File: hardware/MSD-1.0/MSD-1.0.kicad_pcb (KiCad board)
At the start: 2 copper layers, 98.4 x 44.4 mm, 27 parts, among them J1 Conn_01x05, J2 Conn_01x03, Q1 IRF840, U1 NE555P, U2 PC817, U3 PC817

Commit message: new file:   .~BoM.xlsx 	new file:   BoM.xlsx 	new file:   hardware/BoM.xlsx 	deleted:    hardware/MSD-1.0/MSD-1.0-backups/MSD-1.0-2025-03-26_092035.zip 	deleted:    hardware/MSD-1.0/MSD-1.0-backups/MSD-1.0-2025-03-26_092834.zip 	deleted:    hardware/MSD-1.0/MSD-1.0-backups/MSD-1.0-2025-03-27_092014.zip 	new file:   hardware/MSD-1.0/MSD-1.0-backups/MSD-1.0-2025-04-28_130614.zip 	new file:   hardware/MSD-1.0/MSD-1.0-backups/MSD-1.0-2025-04-28_131128.zip 	new file:   hardware/MSD-1.0/MSD-1.0-backups/MSD-1.0-2025-04-28_132753.zip 	new file:   hardware/MSD-1.0/MSD-1.0.csv 	modified:   hardware/MSD-1.0/MSD-1.0.kicad_pcb 	modified:   hardware/MSD-1.0/MSD-1.0.kicad_sch 	deleted:    hardware/PS-1.0/PS-1.0-backups/PS-1.0-2025-03-24_111800.zip 	deleted:    hardware/PS-1.0/PS-1.0-backups/PS-1.0-2025-03-24_112738.zip 	deleted:    hardware/PS-1.0/PS-1.0-backups/PS-1.0-2025-03-25_152833.zip 	deleted:    hardware/PS-1.0/PS-1.0-backups/PS-1.0-2025-03-25_154601.zip 	deleted:    hardware/PS-1.0/PS-1.0-backups/PS-1.0-2025-03-25_155821.zip 	deleted:    hardware/PS-1.0/PS-1.0-backups/PS-1.0-2025-04-11_101418.zip 	deleted:    hardware/PS-1.0/PS-1.0-backups/PS-1.0-2025-04-11_110528.zip 	deleted:    hardware/PS-1.0/PS-1.0-backups/PS-1.0-2025-04-11_111527.zip 	deleted:    hardware/PS-1.0/PS-1.0-backups/PS-1.0-2025-04-11_114252.zip 	deleted:    hardware/PS-1.0/PS-1.0-backups/PS-1.0-2025-04-17_105409.zip 	new file:   hardware/PS-1.0/PS-1.0-backups/PS-1.0-2025-04-19_071925.zip 	new file:   hardware/PS-1.0/PS-1.0-backups/PS-1.0-2025-04-27_222808.zip 	new file:   hardware/PS-1.0/PS-1.0-backups/PS-1.0-2025-04-27_223939.zip 	new file:   hardware/PS-1.0/PS-1.0-backups/PS-1.0-2025-04-27_224445.zip 	new file:   hardware/PS-1.0/PS-1.0-backups/PS-1.0-2025-04-27_225206.zip 	new file:   hardware/PS-1.0/PS-1.0-backups/PS-1.0-2025-04-27_230217.zip 	new file:   hardware/PS-1.0/PS-1.0-backups/PS-1.0-2025-04-28_083014.zip 	new file:   hardware/PS-1.0/PS-1.0-backups/PS-1.0-2025-04-28_112951.zip 	new file:   har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
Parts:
- C1: value 2.2nF -> 2.2nF 100
- C2: value 10nF -> 10nF 63
- C3: value 0.022uF 400V MKP -> 0.022uF 400
- C4: value 100nF -> 100nF 100
- C5: value 100nF 400V -> 100nF 400
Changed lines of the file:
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@@
 			)
 		)
-		(property "Value" "10nF"
+		(property "Value" "10nF 63"
 			(at 2.5 3 0)
 			(layer "F.Fab")
@@
 			)
 		)
-		(property "Value" "0.022uF 400V MKP"
+		(property "Value" "0.022uF 400"
 			(at 5 3.75 0)
 			(layer "F.Fab")
@@
 			)
 		)
-		(property "Value" "100nF 400V"
+		(property "Value" "100nF 400"
 			(at 5 3.75 0)
 			(layer "F.Fab")
@@
 			)
 		)
-		(property "Value" "100nF"
+		(property "Value" "100nF 100"
 			(at 2.5 3 0)
 			(layer "F.Fab")
@@
 			)
 		)
-		(property "Value" "2.2nF"
+		(property "Value" "2.2nF 100"
 			(at 2.5 3 0)
 			(layer "F.Fab")

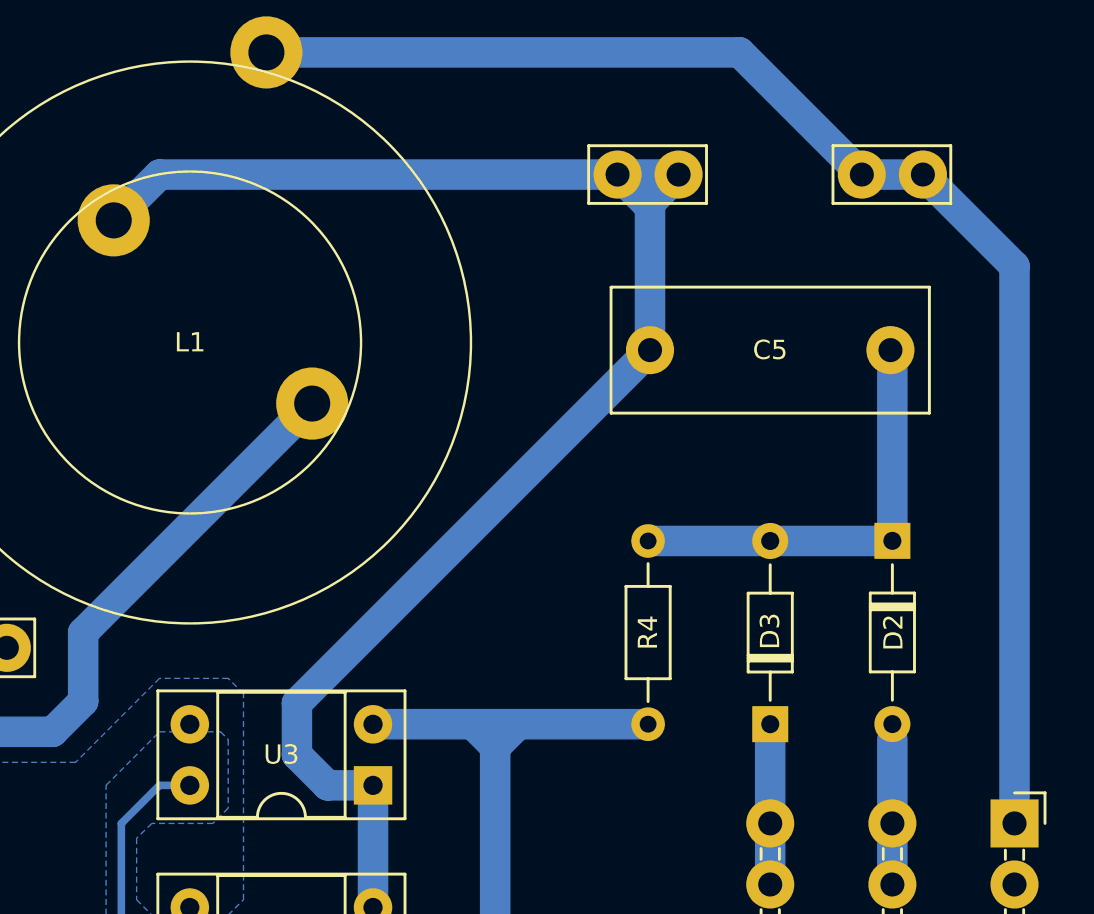
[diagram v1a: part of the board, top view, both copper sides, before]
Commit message: modified:   .DS_Store 	modified:   README.md 	deleted:    hardware/MSD-1.0/MSD-1.0 BoM.csv 	deleted:    hardware/MSD-1.0/MSD-1.0-backups/MSD-1.0-2025-04-08_110759.zip 	deleted:    hardware/MSD-1.0/MSD-1.0-backups/MSD-1.0-2025-04-08_111313.zip 	new file:   hardware/MSD-1.0/MSD-1.0-backups/MSD-1.0-2025-05-06_093009.zip 	new file:   hardware/MSD-1.0/MSD-1.0-backups/MSD-1.0-2025-05-06_093605.zip 	modified:   hardware/MSD-1.0/MSD-1.0.kicad_pcb 	modified:   hardware/MSD-1.0/MSD-1.0.kicad_sch 	modified:   hardware/MSD-1.0/fp-info-cache 	deleted:    hardware/PS-1.0/PS-1.0-backups/PS-1.0-2025-04-16_161300.zip 	deleted:    hardware/PS-1.0/PS-1.0-backups/PS-1.0-2025-04-16_162332.zip 	deleted:    hardware/PS-1.0/PS-1.0-backups/PS-1.0-2025-04-16_163259.zip 	deleted:    hardware/PS-1.0/PS-1.0-backups/PS-1.0-2025-04-17_110908.zip 	deleted:    hardware/PS-1.0/PS-1.0-backups/PS-1.0-2025-04-17_114838.zip 	deleted:    hardware/PS-1.0/PS-1.0-backups/PS-1.0-2025-04-17_155117.zip 	new file:   hardware/PS-1.0/PS-1.0-backups/PS-1.0-2025-05-06_094214.zip 	new file:   hardware/PS-1.0/PS-1.0-backups/PS-1.0-2025-05-06_095559.zip 	new file:   hardware/PS-1.0/PS-1.0-backups/PS-1.0-2025-05-06_100430.zip 	new file:   hardware/PS-1.0/PS-1.0-backups/PS-1.0-2025-05-06_100931.zip 	new file:   hardware/PS-1.0/PS-1.0-backups/PS-1.0-2025-05-06_101736.zip 	new file:   hardware/PS-1.0/PS-1.0-backups/PS-1.0-2025-05-06_102708.zip 	modified:   hardware/PS-1.0/PS-1.0.kicad_pcb 	modified:   hardware/PS-1.0/PS-1.0.kicad_sch 	new file:   hardware/PS-2.0/PS-2.0-B_Cu.gbr 	new file:   hardware/PS-2.0/PS-2.0-B_Mask.gbr 	new file:   hardware/PS-2.0/PS-2.0-B_Paste.gbr 	new file:   hardware/PS-2.0/PS-2.0-B_Silkscreen.gbr 	new file:   hardware/PS-2.0/PS-2.0-Edge_Cuts.gbr 	new file:   hardware/PS-2.0/PS-2.0-F_Cu.gbr 	new file:   hardware/PS-2.0/PS-2.0-F_Mask.gbr 	new file:   hardware/PS-2.0/PS-2.0-F_Paste.gbr 	new file:   hardware/PS-2.0/PS-2.0-F_Silkscreen.gbr 	new file:   hardware/PS-2.0/PS-2.0-NPTH.drl 	new file:   har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
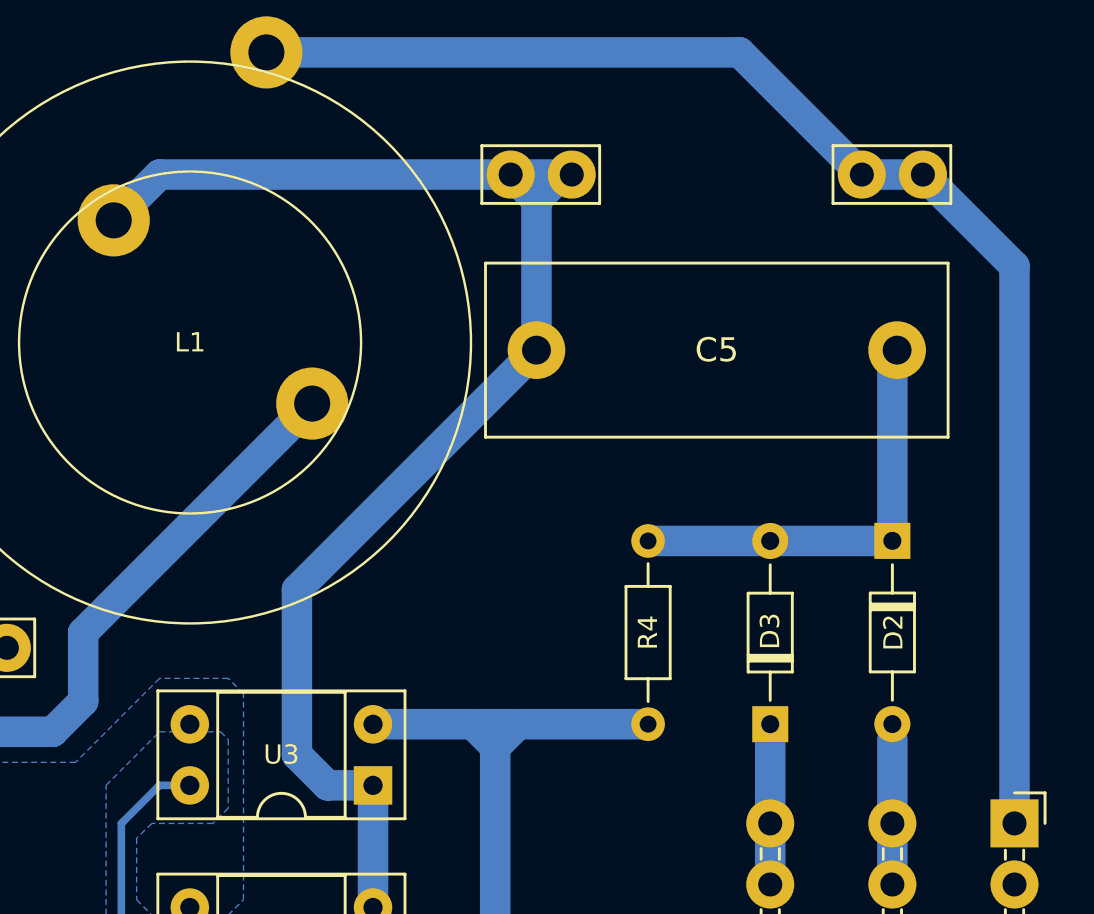
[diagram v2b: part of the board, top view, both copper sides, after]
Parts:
- C3: value 0.022uF 400 -> 0.022µF 400
- C5: value 100nF 400 -> 0.1µF 400; footprint Capacitor_THT:C_Rect_L13.0mm_W5.0mm_P10.00mm_FKS3_FKP3_MKS4 -> Capacitor_THT:C_Rect_L19.0mm_W7.0mm_P15.00mm_MKS4
- moved C5 4.72 mm to (141.1, 40.3)
- moved TP3 4.44 mm to (140.0, 33.0)
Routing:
- net Net-(C5-Pad1): track 65.7 -> 59.2 mm
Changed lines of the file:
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@@
 	(footprint "TestPoint:TestPoint_Bridge_Pitch2.54mm_Drill1.0mm"
 		(layer "F.Cu")
-		(at 144.4625 33.02)
+		(at 140.0175 33.02)
 		(descr "wire loop as test point, pitch 2.54mm, hole diameter 1.0mm, wire diameter 0.8mm")
 		(tags "test point wire loop")
@@
 			)
 		)
-		(property "Value" "0.022uF 400"
+		(property "Value" "0.022µF 400"
 			(at 5 3.75 0)
 			(layer "F.Fab")
@@
 		)
 	)
-	(footprint "Capacitor_THT:C_Rect_L13.0mm_W5.0mm_P10.00mm_FKS3_FKP3_MKS4"
+	(footprint "Capacitor_THT:C_Rect_L19.0mm_W7.0mm_P15.00mm_MKS4"
 		(layer "F.Cu")
-		(at 145.8125 40.3225)
-		(descr "C, Rect series, Radial, pin pitch=10.00mm, , length*width=13*5mm^2, Capacitor, http://www.wima.com/EN/WIMA_FKS_3.pdf, http://www.wima.com/EN/WIMA_MKS_4.pdf")
-		(tags "C Rect series Radial pin pitch 10.00mm  length 13mm width 5mm Capacitor")
+		(at 141.09 40.3225)
+		(descr "C, Rect series, Radial, pin pitch=15.00mm, , length*width=19*7mm^2, Capacitor, http://www.wima.com/EN/WIMA_MKS_4.pdf")
+		(tags "C Rect series Radial pin pitch 15.00mm  length 19mm width 7mm Capacitor")
 		(property "Reference" "C5"
-			(at 5 0 0)
+			(at 7.5 0 0)
 			(layer "F.SilkS")
 			(effects
 				(font
-					(size 0.8 0.8)
+					(size 1 1)
 					(thickness 0.15)
 				)
 			)
 		)
-		(property "Value" "100nF 400"
-			(at 5 3.75 0)
+		(property "Value" "0.1µF 400"
+			(at 7.5 4.75 0)
 			(layer "F.Fab")
 			(effects
@@
 			)
 		)
-		(property "Footprint" "Capacitor_THT:C_Rect_L13.0mm_W5.0mm_P10.00mm_FKS3_FKP3_MKS4"
+		(property "Footprint" "Capacitor_THT:C_Rect_L19.0mm_W7.0mm_P15.00mm_MKS4"
 			(at 0 0 0)
 			(unlocked yes)
@@
 		(attr through_hole)
 		(fp_line
-			(start -1.62 -2.62)
-			(end -1.62 2.62)
+			(start -2.12 -3.62)
+			(end -2.12 3.62)
 			(stroke
 				(width 0.12)
@@
 		)
 		(fp_line
-			(start -1.62 -2.62)
-			(end 11.62 -2.62)
+			(start -2.12 -3.62)
+			(end 17.12 -3.62)
 			(stroke
 				(width 0.12)
@@
 		)
 		(fp_line
-			(start -1.62 2.62)
-			(end 11.62 2.62)
+			(start -2.12 3.62)
+			(end 17.12 3.62)
 			(stroke
 				(width 0.12)
@@
 		)
 		(fp_line
-			(start 11.62 -2.62)
-			(end 11.62 2.62)
+			(start 17.12 -3.62)
+			(end 17.12 3.62)
 			(stroke
 				(width 0.12)
@@
 		)
 		(fp_line
-			(start -1.75 -2.75)
-			(end -1.75 2.75)
+			(start -2.25 -3.75)
+			(end -2.25 3.75)
 			(stroke
 				(width 0.05)
@@
 		)
 		(fp_line
-			(start -1.75 2.75)
-			(end 11.75 2.75)
+			(start -2.25 3.75)
+			(end 17.25 3.75)
 			(stroke
 				(width 0.05)
@@
 		)
 		(fp_line
-			(start 11.75 -2.75)
-			(end -1.75 -2.75)
+			(start 17.25 -3.75)
+			(end -2.25 -3.75)
 			(stroke
 				(width 0.05)
@@
 		)
 		(fp_line
-			(start 11.75 2.75)
-			(end 11.75 -2.75)
+			(start 17.25 3.75)
+			(end 17.25 -3.75)
 			(stroke
 				(width 0.05)
@@
 		)
 		(fp_line
-			(start -1.5 -2.5)
-			(end -1.5 2.5)
+			(start -2 -3.5)
+			(end -2 3.5)
 			(stroke
 				(width 0.1)
@@
 		)
 		(fp_line
-			(start -1.5 2.5)
-			(end 11.5 2.5)
+			(start -2 3.5)
+			(end 17 3.5)
 			(stroke
 				(width 0.1)
@@
 		)
 		(fp_line
-			(start 11.5 -2.5)
-			(end -1.5 -2.5)
+			(start 17 -3.5)
+			(end -2 -3.5)
 			(stroke
 				(width 0.1)
@@
 		)
 		(fp_line
-			(start 11.5 2.5)
-			(end 11.5 -2.5)
+			(start 17 3.5)
+			(end 17 -3.5)
 			(stroke
 				(width 0.1)
@@
 		)
 		(fp_text user "${REFERENCE}"
-			(at 5 0 0)
+			(at 7.5 0 0)
 			(layer "F.Fab")
 			(effects
@@
 		(pad "1" thru_hole circle
 			(at 0 0)
-			(size 2 2)
-			(drill 1)
+			(size 2.4 2.4)
+			(drill 1.2)
 			(layers "*.Cu" "*.Mask")
 			(remove_unused_layers no)
@@
 		)
 		(pad "2" thru_hole circle
-			(at 10 0)
-			(size 2 2)
-			(drill 1)
+			(at 15 0)
+			(size 2.4 2.4)
+			(drill 1.2)
 			(layers "*.Cu" "*.Mask")
 			(remove_unused_layers no)
@@
 			(pintype "passive")
 		)
-		(model "${KICAD8_3DMODEL_DIR}/Capacitor_THT.3dshapes/C_Rect_L13.0mm_W5.0mm_P10.00mm_FKS3_FKP3_MKS4.wrl"
+		(model "${KICAD8_3DMODEL_DIR}/Capacitor_THT.3dshapes/C_Rect_L19.0mm_W7.0mm_P15.00mm_MKS4.wrl"
 			(offset
 				(xyz 0 0 0)
@@
 	)
 	(segment
-		(start 145.8125 34.37)
-		(end 144.4625 33.02)
+		(start 141.09 34.0925)
+		(end 140.0175 33.02)
 		(width 1.27)
 		(layer "B.Cu")
@@
 	)
 	(segment
-		(start 131.1275 57.15)
-		(end 131.1275 55.0075)
+		(start 131.1275 50.285)
+		(end 141.09 40.3225)
 		(width 1.27)
 		(layer "B.Cu")
@@
 	)
 	(segment
-		(start 145.8125 34.37)
-		(end 145.8125 34.21)
+		(start 142.1625 33.02)
+		(end 141.09 34.0925)
 		(width 1.27)
 		(layer "B.Cu")
@@
 	)
 	(segment
-		(start 147.0025 33.02)
-		(end 144.4625 33.02)
+		(start 131.1275 57.15)
+		(end 132.4025 58.425)
 		(width 1.27)
 		(layer "B.Cu")
@@
 	)
 	(segment
-		(start 131.1275 57.15)
-		(end 132.4025 58.425)
+		(start 142.5575 33.02)
+		(end 142.1625 33.02)
 		(width 1.27)
 		(layer "B.Cu")
@@
 	(segment
 		(start 125.4125 33.02)
-		(end 144.4625 33.02)
+		(end 140.0175 33.02)
 		(width 1.27)
 		(layer "B.Cu")
@@
 	)
 	(segment
-		(start 145.8125 40.3225)
-		(end 145.8125 34.37)
+		(start 140.0175 33.02)
+		(end 142.5575 33.02)
 		(width 1.27)
 		(layer "B.Cu")
@@
 	)
 	(segment
-		(start 132.4025 58.425)
-		(end 134.2925 58.425)
+		(start 141.09 40.3225)
+		(end 141.09 34.0925)
 		(width 1.27)
 		(layer "B.Cu")
@@
 	)
 	(segment
-		(start 123.5075 34.925)
-		(end 125.4125 33.02)
+		(start 132.4025 58.425)
+		(end 134.2925 58.425)
 		(width 1.27)
 		(layer "B.Cu")
@@
 	)
 	(segment
-		(start 131.1275 55.0075)
-		(end 145.8125 40.3225)
+		(start 123.5075 34.925)
+		(end 125.4125 33.02)
 		(width 1.27)
 		(layer "B.Cu")
@@
 	)
 	(segment
-		(start 145.8125 34.21)
-		(end 147.0025 33.02)
+		(start 131.1275 57.15)
+		(end 131.1275 50.285)
 		(width 1.27)
 		(layer "B.Cu")
@@
 	(segment
 		(start 155.8925 48.255)
-		(end 155.8925 40.4025)
+		(end 155.8925 40.52)
+		(width 1.27)
+		(layer "B.Cu")
+		(net 12)
+	)
+	(segment
+		(start 155.8925 40.52)
+		(end 156.09 40.3225)
 		(width 1.27)
 		(layer "B.Cu")
